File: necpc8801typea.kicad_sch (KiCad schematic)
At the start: 263 parts, among them J2 Conn_01x04_MountingPin, Q1 Q_PMOS_GSD AO3401A, Q2 Q_NMOS_GSD 2N7002, Q3 Q_NMOS_GSD 2N7002, Q4 2N3904, SW1 SW_Push, U1 AMS1117-3.3, U2 TPS2553DBVR, U3 STM32F401RETx, U4 24LC64, U5 USBLC6-2SC6, Y1 8MHz

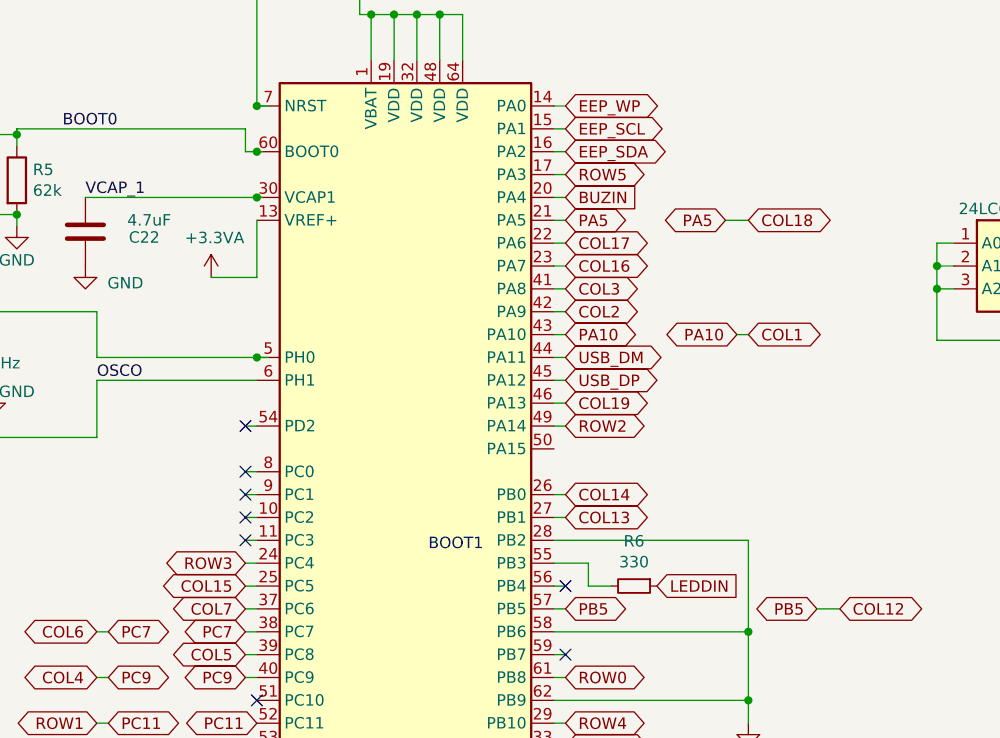
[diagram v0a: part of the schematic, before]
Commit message: cleanup
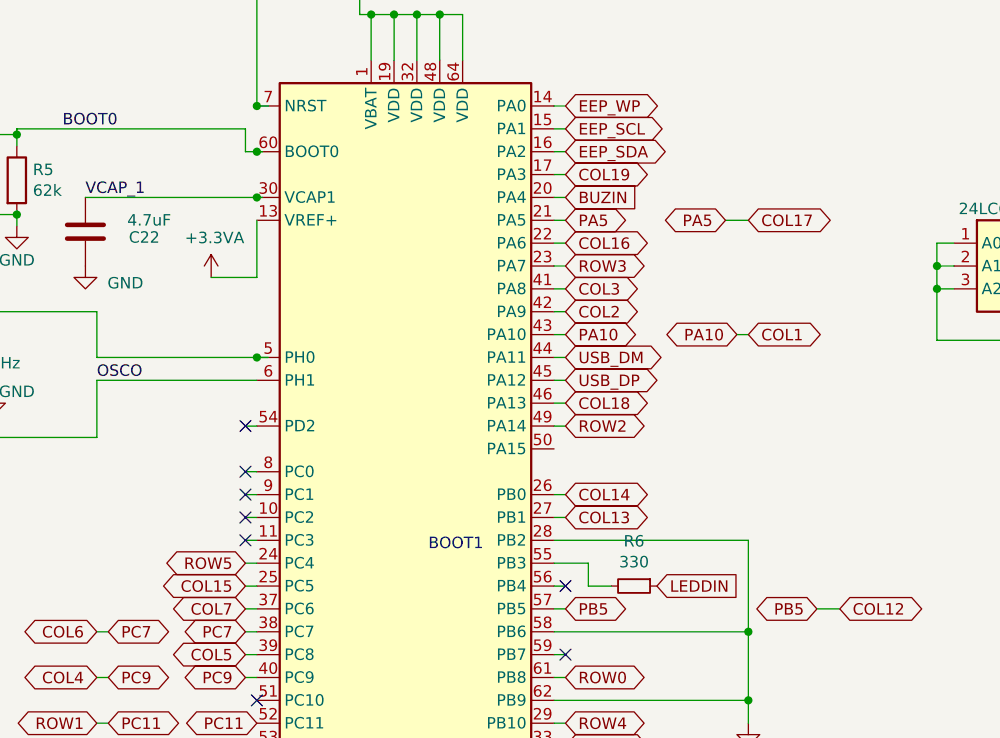
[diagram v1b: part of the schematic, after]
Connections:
- net COL16: now also U3.22 (PA6); no longer U3.23 (PA7)
- net COL17: now also R13.2, U3.21 (PA5); no longer U3.22 (PA6)
- net COL18: now also U3.46 (PA13); no longer R13.2, U3.21 (PA5)
- net COL19: now also U3.17 (PA3); no longer U3.46 (PA13)
- net ROW3: now also U3.23 (PA7); no longer U3.24 (PC4)
- net ROW5: now also U3.24 (PC4); no longer U3.17 (PA3)

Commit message: updates
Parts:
- removed C4, C5, C7: 100nF, Capacitor_SMD:C_0805_2012Metric_Pad1.18x1.45mm_HandSolder, symbol Device:C
- removed C6, C9: 22uF, Capacitor_SMD:C_0805_2012Metric_Pad1.18x1.45mm_HandSolder, symbol Device:C
- removed R1, R13: 62k, Resistor_SMD:R_0805_2012Metric_Pad1.20x1.40mm_HandSolder, symbol Device:R
- removed U2: TPS2553DBVR, Package_TO_SOT_SMD:SOT-23-6_Handsoldering, symbol tps2553dbvr:TPS2553DBVR
- added R18, R19: 62k, Resistor_SMD:R_0805_2012Metric_Pad1.20x1.40mm_HandSolder, symbol Device:R
- C8: value 100nF -> 1uF
- U1: value AMS1117-3.3 -> XC6206P332NR
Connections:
- net +3.3VA: now also R16.1, R17.1, R18.1, R19.1
- net +5V: now also C3.1, FB1.1
- net COL1: now also R12.2; no longer R15.2
- net COL10: now also R18.2
- net COL12: no longer R17.2
- net COL17: now also R17.2
- net COL4: no longer R12.2
- net COL6: no longer R14.2
- net EEP_SCL: now also U3.61 (PB8); no longer U3.15 (PA1)
- net EEP_SDA: now also U3.62 (PB9); no longer U3.16 (PA2)
- net GND: no longer R16.1, R17.1, U3.58 (PB6), U3.62 (PB9)
- net ROW0: now also U3.24 (PC4); no longer U3.61 (PB8)
- net ROW5: now also U3.15 (PA1); no longer U3.24 (PC4)
- net PB3: now reaches R6.2, U3.55 (PB3)
- net PB3: now also R15.2
- net PC10: now reaches U3.51 (PC10)
- net PC10: now also R19.2
- net PB4: now reaches U3.56 (PB4)
- net PB4: now also R16.2
- net PB7: now reaches U3.59 (PB7)
- net PB7: now also R14.2
- net PC11 renamed ROW1
- net ROW1: no longer R16.2
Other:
- note added: "These are all pulled up to disable all non-DFU bootloader modes"
- moved on the sheet: BUZ1, C16, C17, C18, C21, C3, C8, LED1, LED2, LED3, Q4, R10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
